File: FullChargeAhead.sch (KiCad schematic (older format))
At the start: 18 parts, among them P101 CONN_01X02, P102 JST 2 Pin, U101 MCP73834-FCI/UN

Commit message: Started BOM
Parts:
- C101: ConradPN (none) -> 1278977 - 62
- C102: ConradPN (none) -> 1278977 - 62; MPN (none) -> Value
- D101: ConradPN (none) -> N/A; MPN (none) -> N/A
- D102, D103: ConradPN (none) -> 180102 - 62; MPN (none) -> KP-2012EC
- U101: ConradPN (none) -> 1085505 - 62; MPN (none) -> MCP73834-FCI/UN
- USB1: ConradPN (none) -> N/A; MPN Value -> 10118193-0001LF
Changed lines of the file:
@@
 F 2 "Housings_SSOP:MSOP-10_3x3mm_Pitch0.5mm" H 6700 3350 60  0001 C CNN
 F 3 "" H 6700 3350 60  0000 C CNN
+F 4 "MCP73834-FCI/UN" H 6900 3350 60  0001 C CNN "MPN"
+F 5 "1085505 - 62 " H 6900 3350 60  0001 C CNN "ConradPN"
 	1    6900 3350
 	1    0    0    -1
@@
 F 2 "LEDs:LED-0805" H 4350 3250 60  0001 C CNN
 F 3 "" H 4350 3250 60  0000 C CNN
+F 4 "N/A" H 4350 3250 60  0001 C CNN "MPN"
+F 5 "N/A" H 4350 3250 60  0001 C CNN "ConradPN"
 	1    4350 3250
 	0    1    1    0
@@
 F 2 "LEDs:LED-0805" H 4800 3250 60  0001 C CNN
 F 3 "" H 4800 3250 60  0000 C CNN
+F 4 "KP-2012EC" H 4800 3250 60  0001 C CNN "MPN"
+F 5 "180102 - 62" H 4800 3250 60  0001 C CNN "ConradPN"
 	1    4800 3250
 	0    1    1    0
@@
 F 2 "LEDs:LED-0805" H 5200 3250 60  0001 C CNN
 F 3 "" H 5200 3250 60  0000 C CNN
+F 4 "KP-2012EC" H 5200 3250 60  0001 C CNN "MPN"
+F 5 "180102 - 62" H 5200 3250 60  0001 C CNN "ConradPN"
 	1    5200 3250
 	0    1    1    0
@@
 F 3 "" H 3700 3250 60  0000 C CNN
 F 4 "Value" H 3700 3250 60  0001 C CNN "MPN"
+F 5 "1278977 - 62" H 3700 3250 60  0001 C CNN "ConradPN"
 	1    3700 3250
 	1    0    0    -1
@@
 F 2 "Capacitors_SMD:C_1206_HandSoldering" H 8938 3100 30  0001 C CNN
 F 3 "" H 8900 3250 60  0000 C CNN
+F 4 "Value" H 8900 3250 60  0001 C CNN "MPN"
+F 5 "1278977 - 62" H 8900 3250 60  0001 C CNN "ConradPN"
 	1    8900 3250
 	1    0    0    -1
@@
 F 2 "fca-lib:USB_Micro_B" H 2700 2600 50  0001 C CNN
 F 3 "" H 2700 2600 50  0000 C CNN
-F 4 "Value" H 2700 2700 60  0001 C CNN "MPN"
+F 4 "10118193-0001LF" H 2700 2700 60  0001 C CNN "MPN"
+F 5 "N/A" H 2700 2700 60  0001 C CNN "ConradPN"
 	1    2700 2700
 	-1   0    0    1

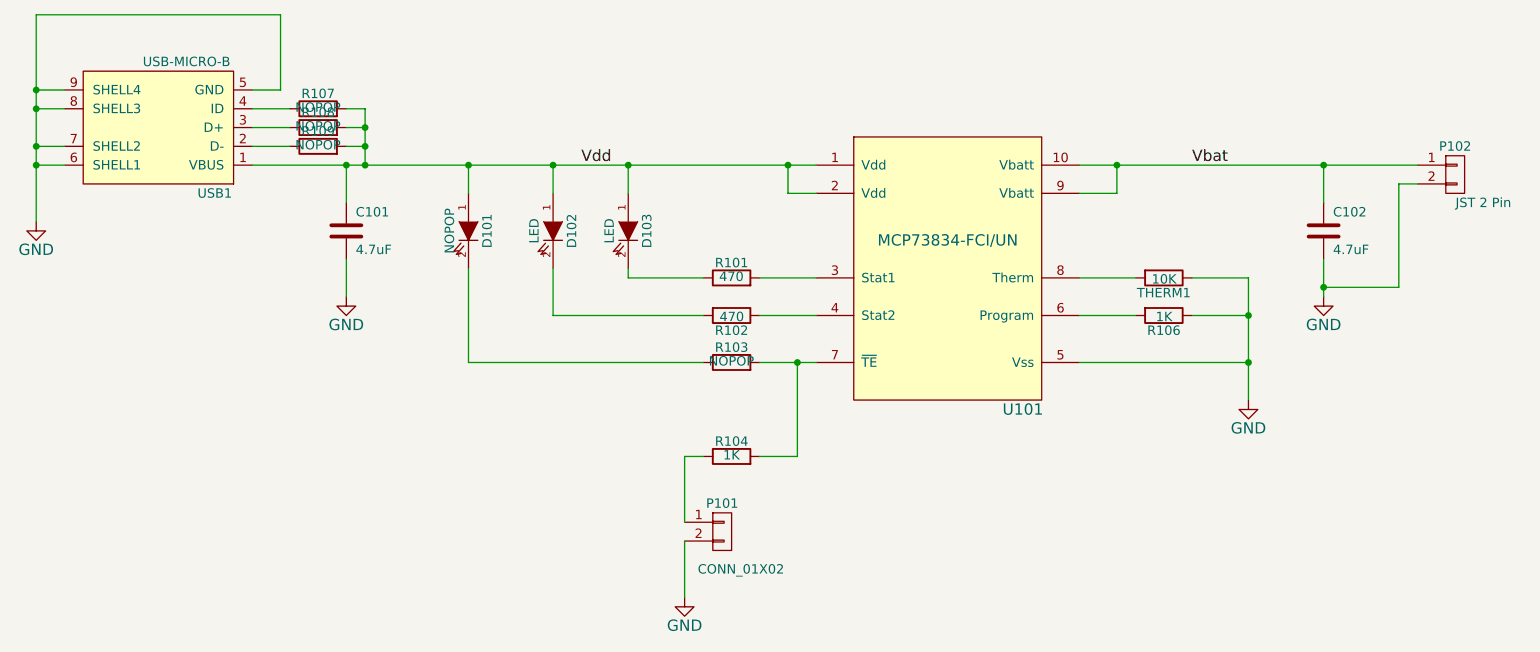
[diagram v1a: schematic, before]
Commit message: Some changes and test results
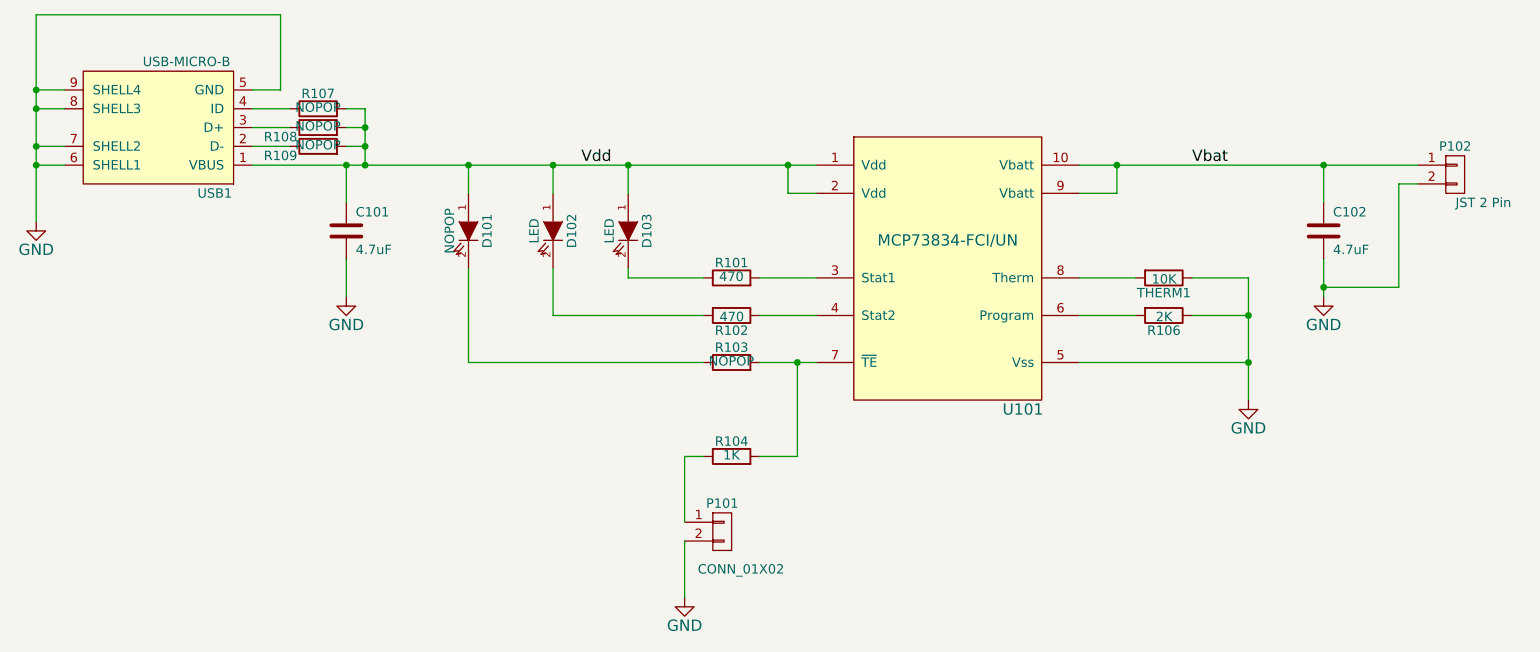
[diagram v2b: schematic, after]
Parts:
- R106: value 1K -> 2K
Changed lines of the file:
@@
 P 8050 3700
 F 0 "R106" V 8130 3700 50  0000 C CNN
-F 1 "1K" V 8057 3701 50  0000 C CNN
+F 1 "2K" V 8057 3701 50  0000 C CNN
 F 2 "Resistors_SMD:R_0805_HandSoldering" V 7980 3700 30  0001 C CNN
 F 3 "" H 8050 3700 30  0000 C CNN
@@
 U 1 1 55106F74
 P 3550 2700
-F 0 "R108" V 3630 2700 50  0000 C CNN
+F 0 "R108" V 3500 2900 50  0000 C CNN
 F 1 "NOPOP" V 3557 2701 50  0000 C CNN
 F 2 "Resistors_SMD:R_0805_HandSoldering" V 3480 2700 30  0001 C CNN
@@
 U 1 1 55106FB8
 P 3550 2800
-F 0 "R109" V 3630 2800 50  0000 C CNN
+F 0 "R109" V 3500 3000 50  0000 C CNN
 F 1 "NOPOP" V 3557 2801 50  0000 C CNN
 F 2 "Resistors_SMD:R_0805_HandSoldering" V 3480 2800 30  0001 C CNN

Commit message: Updated the documentation
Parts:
- D101, D102, D103: symbol LED -> LED-RESCUE-FullChargeAhead
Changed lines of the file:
@@
 EESchema Schematic File Version 2
+LIBS:FullChargeAhead-rescue
 LIBS:power
 LIBS:device
@@
 LIBS:memory
 LIBS:xilinx
-LIBS:special
 LIBS:microcontrollers
 LIBS:dsp
@@
 $EndComp
 $Comp
-L LED D101
+L LED-RESCUE-FullChargeAhead D101
 U 1 1 550DA792
 P 4350 3250
@@
 $EndComp
 $Comp
-L LED D102
+L LED-RESCUE-FullChargeAhead D102
 U 1 1 550DA80B
 P 4800 3250
@@
 $EndComp
 $Comp
-L LED D103
+L LED-RESCUE-FullChargeAhead D103
 U 1 1 550DA883
 P 5200 3250
